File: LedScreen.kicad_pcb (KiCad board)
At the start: 2 copper layers, 85 x 88.5 mm, 42 parts

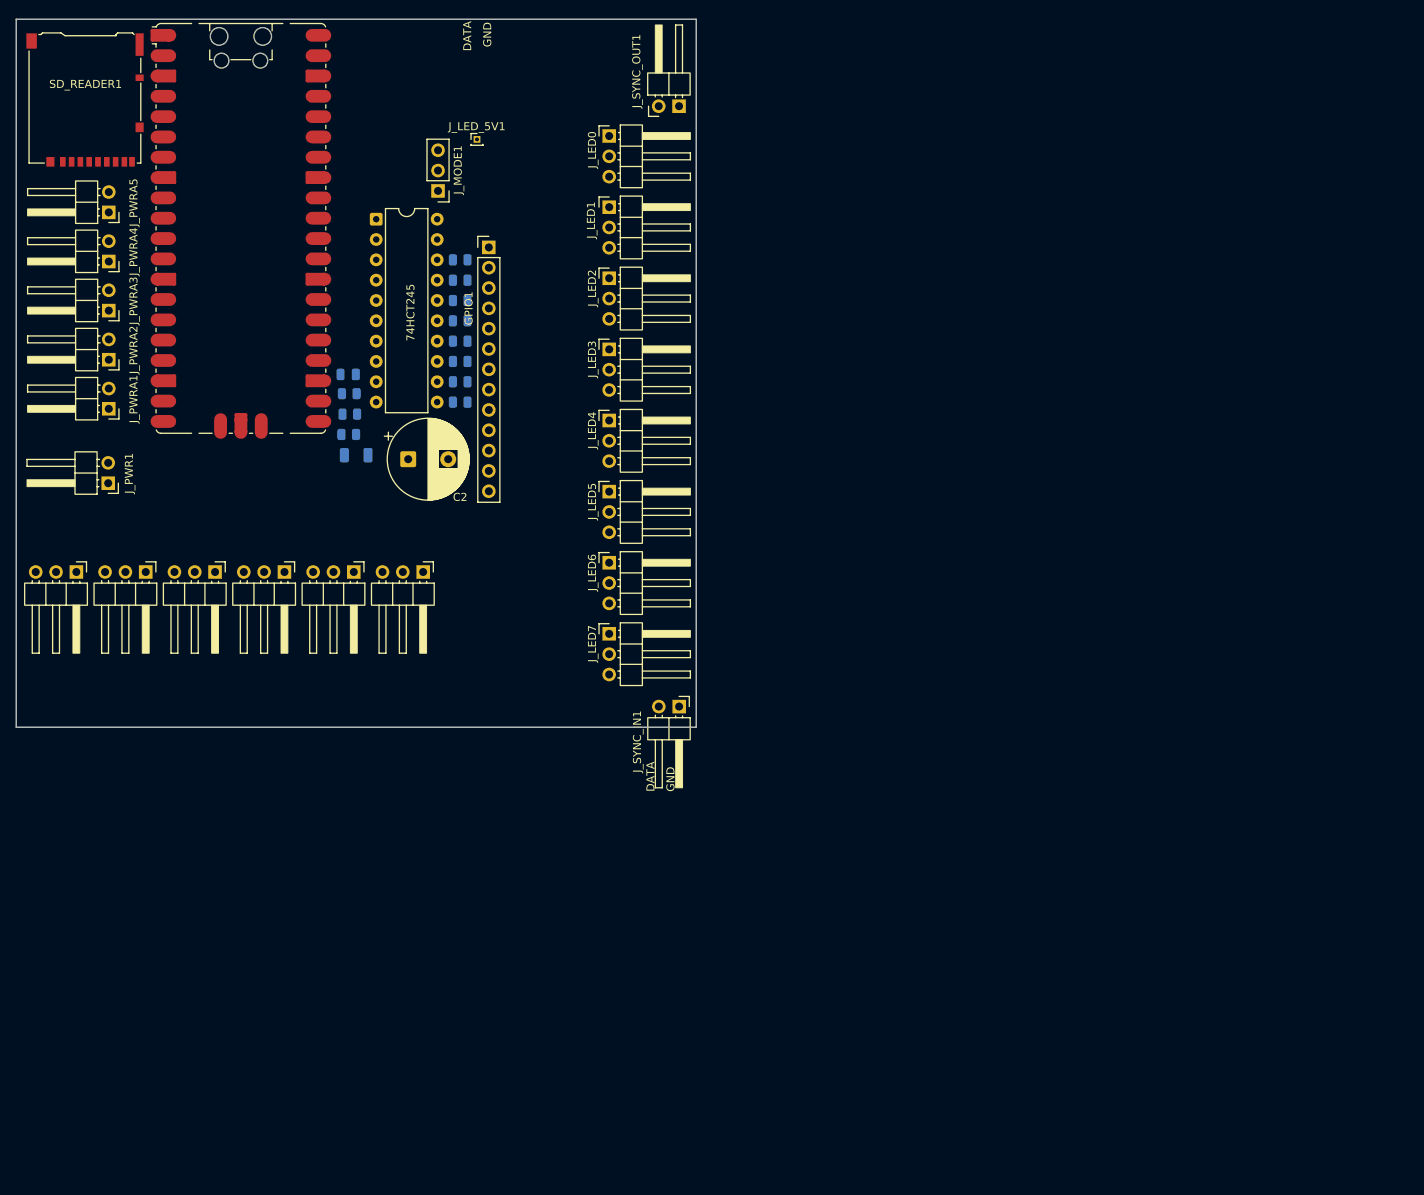
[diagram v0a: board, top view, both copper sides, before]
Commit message: finsighed new v2 routing
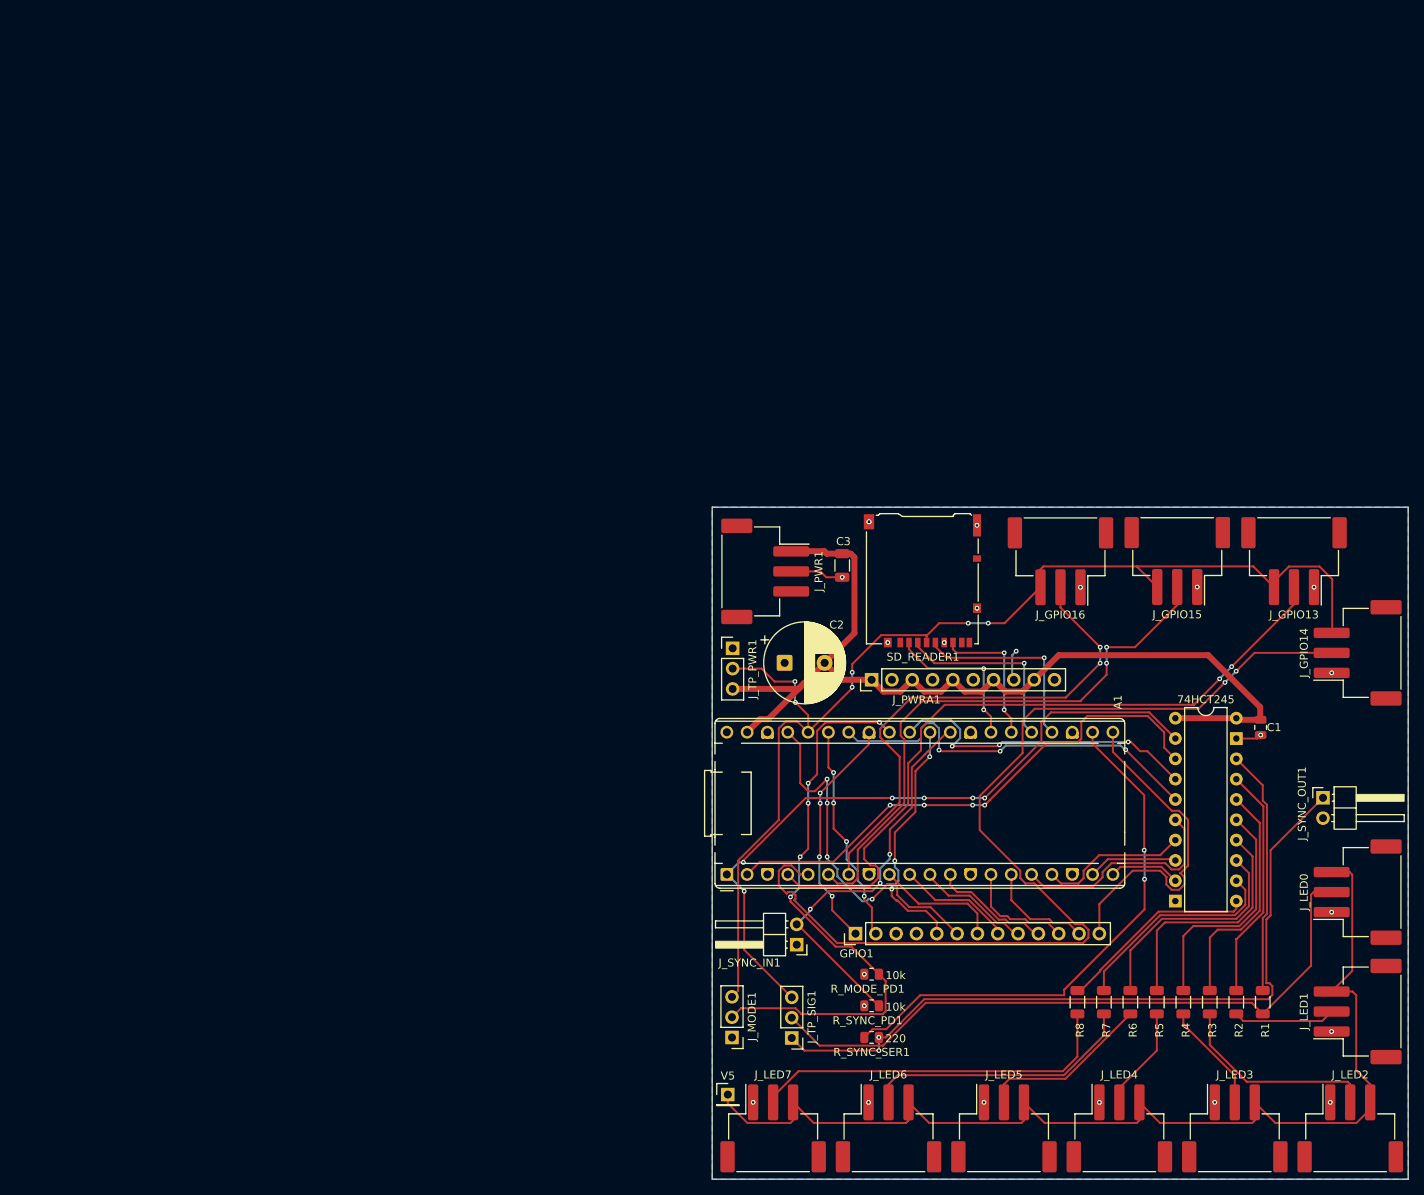
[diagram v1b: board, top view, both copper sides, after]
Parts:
- removed J_LED_5V1: Conn_01x01_Pin, Connector_PinHeader_1.00mm:PinHeader_1x01_P1.00mm_Vertical
- removed J_PWRA2, J_PWRA3, J_PWRA4, J_PWRA5: Conn_01x02, Connector_PinHeader_2.54mm:PinHeader_1x02_P2.54mm_Horizontal
- added V5: Conn_01x01_Pin, Connector_PinHeader_2.54mm:PinHeader_1x01_P2.54mm_Vertical, F.Cu at (88.9, 134.4)
- A1: footprint Module:RaspberryPi_Pico_SMD_HandSolder -> Module:RaspberryPi_Pico_Common_THT
- C1, C3, R_MODE_PD1, R_SYNC_PD1, R_SYNC_SER1: moved to F.Cu
- J_GPIO13, J_GPIO14, J_GPIO15, J_GPIO16, J_LED0, J_LED1, J_LED2, J_LED3, J_LED4, J_LED5, J_LED6, J_LED7: footprint Connector_PinHeader_2.54mm:PinHeader_1x03_P2.54mm_Horizontal -> Connector_JST:JST_XH_S3B-XH-SM4-TB_1x03-1MP_P2.50mm_Horizontal
- J_PWR1: value Conn_01x02 -> Conn_01x03; footprint Connector_PinHeader_2.54mm:PinHeader_1x02_P2.54mm_Horizontal -> Connector_JST:JST_XH_S3B-XH-SM4-TB_1x03-1MP_P2.50mm_Horizontal
- J_PWRA1: value Conn_01x02 -> Conn_01x10; footprint Connector_PinHeader_2.54mm:PinHeader_1x02_P2.54mm_Horizontal -> Connector_PinHeader_2.54mm:PinHeader_1x10_P2.54mm_Vertical
- J_TP_PWR1, J_TP_SIG1: footprint Connector_PinHeader_2.54mm:PinHeader_1x03_P2.54mm_Horizontal -> Connector_PinHeader_2.54mm:PinHeader_1x03_P2.54mm_Vertical
- R1, R2, R3, R4, R5, R6, R7, R8: value 330 (0-330) -> 0R; footprint Resistor_SMD:R_0805_2012Metric -> Resistor_SMD:R_1206_3216Metric; moved to F.Cu
- moved J_LED2 141.0 mm to (166.8, 138.6)
- moved J_LED1 137.3 mm to (167.7, 124.0), turned to 90 degrees
- moved R1 136.7 mm to (155.8, 122.9), turned to -90 degrees
- moved J_LED0 133.0 mm to (167.7, 109.1), turned to 90 degrees
- moved R2 132.5 mm to (152.5, 122.9), turned to -90 degrees
- moved R3 128.3 mm to (149.2, 122.9), turned to -90 degrees
- moved J_GPIO14 125.9 mm to (167.7, 79.2), turned to 90 degrees
- moved J_LED3 124.9 mm to (152.3, 138.6)
- moved R4 124.2 mm to (145.9, 122.9), turned to -90 degrees
- moved C1 122.3 mm to (155.6, 88.5), turned to -90 degrees
- moved SD_READER1 120.7 mm to (113.3, 70.2)
- moved R5 120.0 mm to (142.6, 122.9), turned to -90 degrees
- moved J_SYNC_OUT1 119.9 mm to (163.3, 97.3), turned to 0 degrees
- moved 74HCT245 117.8 mm to (144.9, 87.4)
- moved R6 115.9 mm to (139.3, 122.9), turned to -90 degrees
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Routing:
- net +3V3: track 0.00 -> 147.7 mm, vias 0 -> 6
- net LED_PIN3: track 0.00 -> 137.0 mm
- net GPIO3: track 0.00 -> 127.3 mm, vias 0 -> 2
- net +5V: track 0.00 -> 122.2 mm
- net SYNC_OUT: track 0.00 -> 92.8 mm, vias 0 -> 2
- net GPIO2: track 0.00 -> 90.6 mm, vias 0 -> 2
- net T_OUT0: track 0.00 -> 86.6 mm, vias 0 -> 6
- net LED0_DATA: track 0.00 -> 83.2 mm
- net MODE: track 0.00 -> 72.6 mm, vias 0 -> 5
- net GPIO4: track 0.00 -> 71.5 mm, vias 0 -> 2
- net SYNC_OUT_DRV: track 0.00 -> 66.9 mm, vias 0 -> 2
- net T_OUT1: track 0.00 -> 66.3 mm, vias 0 -> 4
- net GPIO5: track 0.00 -> 64.3 mm, vias 0 -> 2
- net SYNC_IN: track 0.00 -> 49.9 mm, vias 0 -> 3
- net T_OUT3: track 0.00 -> 49.1 mm, vias 0 -> 3
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- added copper zone on B.Cu, net GND
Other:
- board size 85 x 88.5 mm -> 87 x 84 mm
- board text removed: "DATA"
- board text removed: "GND"
